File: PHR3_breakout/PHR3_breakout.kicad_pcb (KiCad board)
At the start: 2 copper layers, 11.5 x 17.5 mm, 2 parts, among them J1 Conn_01x03, J2 Conn_01x03

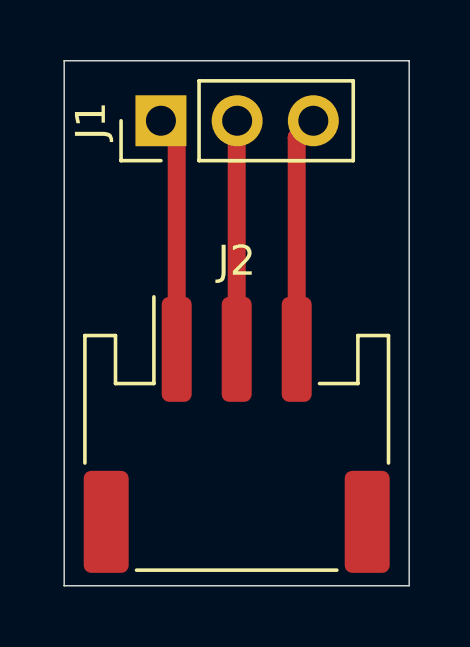
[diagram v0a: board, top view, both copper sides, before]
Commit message: Minor changes
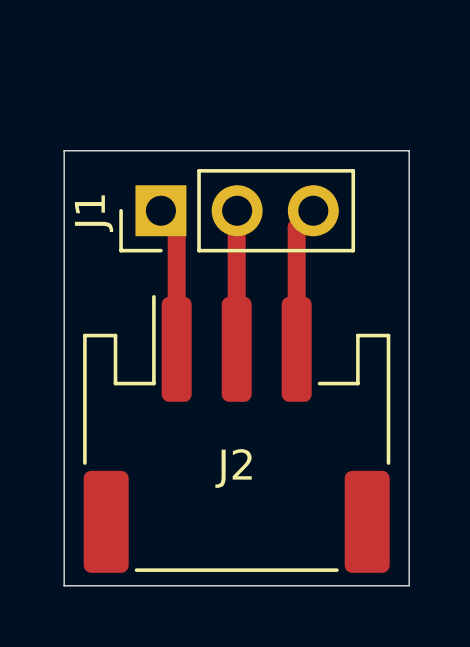
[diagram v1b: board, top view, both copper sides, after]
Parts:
- moved J1 3.00 mm to (146.7, 74.8)
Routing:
- net Net-(J1-Pin_2): track 7.65 -> 4.63 mm
- net Net-(J1-Pin_3): track 7.85 -> 4.85 mm
- net Net-(J1-Pin_1): track 7.84 -> 4.84 mm
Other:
- board size 11.5 x 17.5 mm -> 11.5 x 14.5 mm
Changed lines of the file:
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@@
 		(tags "connector JST PH horizontal")
 		(property "Reference" "J2"
-			(at 0 -5.8 0)
+			(at 0 1.03 0)
 			(layer "F.SilkS")
 			(effects
@@
 	(footprint "Connector_PinHeader_2.54mm:PinHeader_1x03_P2.54mm_Vertical"
 		(layer "F.Cu")
-		(at 146.725 71.75 90)
+		(at 146.725 74.75 90)
 		(descr "Through hole straight pin header, 1x03, 2.54mm pitch, single row")
 		(tags "Through hole pin header THT 1x03 2.54mm single row")
 		(property "Reference" "J1"
-			(at 0 -2.33 270)
+			(at 0 -2.33 -90)
 			(layer "F.SilkS")
 			(effects
@@
 		)
 		(property "Value" "Conn_01x03"
-			(at 0 7.41 270)
+			(at 0 7.41 -90)
 			(layer "F.Fab")
 			(effects
@@
 		)
 		(fp_text user "${REFERENCE}"
-			(at 0 2.54 360)
+			(at 0 2.54 0)
 			(layer "F.Fab")
 			(effects
@@
 	)
 	(gr_rect
-		(start 143.5 69.75)
+		(start 143.5 72.75)
 		(end 155 87.25)
 		(stroke
@@
 	)
 	(segment
-		(start 149.25 79.37)
-		(end 149.25 71.765)
+		(start 149.25 74.765)
+		(end 149.265 74.75)
 		(width 0.6)
 		(layer "F.Cu")
@@
 	)
 	(segment
-		(start 149.2425 71.765)
-		(end 149.2575 71.75)
+		(start 149.25 79.37)
+		(end 149.25 74.765)
 		(width 0.6)
 		(layer "F.Cu")
@@
 	)
 	(segment
-		(start 149.25 71.765)
-		(end 149.265 71.75)
-		(width 0.6)
-		(layer "F.Cu")
-		(net 1)
-	)
-	(segment
-		(start 147.25 79.37)
-		(end 147.25 72.275)
+		(start 147.25 75.275)
+		(end 146.725 74.75)
 		(width 0.6)
 		(layer "F.Cu")
@@
 	)
 	(segment
-		(start 147.25 72.275)
-		(end 146.725 71.75)
+		(start 147.25 79.37)
+		(end 147.25 75.275)
 		(width 0.6)
 		(layer "F.Cu")
@@
 	(segment
 		(start 151.25 79.37)
-		(end 151.25 72.305)
+		(end 151.25 75.305)
 		(width 0.6)
 		(layer "F.Cu")
@@
 	)
 	(segment
-		(start 151.25 72.305)
-		(end 151.805 71.75)
+		(start 151.25 75.305)
+		(end 151.805 74.75)
 		(width 0.6)
 		(layer "F.Cu")
